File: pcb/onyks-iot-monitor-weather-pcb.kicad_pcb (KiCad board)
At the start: 2 copper layers, 100 x 82 mm, 45 parts, among them J1 53398-0371, J10 Conn_01x02_Pin, J11 Conn_01x06_Pin, J12 Conn_02x05_Odd_Even, J13 Conn_01x02_Pin, J2 53398-0371, J3 53048-0810, J3 Conn_01x04_Pin, J4 53398-0371, J5 53398-0371, J6 53398-0371, J7 53398-0371, J8 53398-0371, J9 53398-0371, Q1 SS8050, Q2 SS8050, U1 ESP32-WROOM-32D, U3 TLV75733PDBV, U6 BMP280

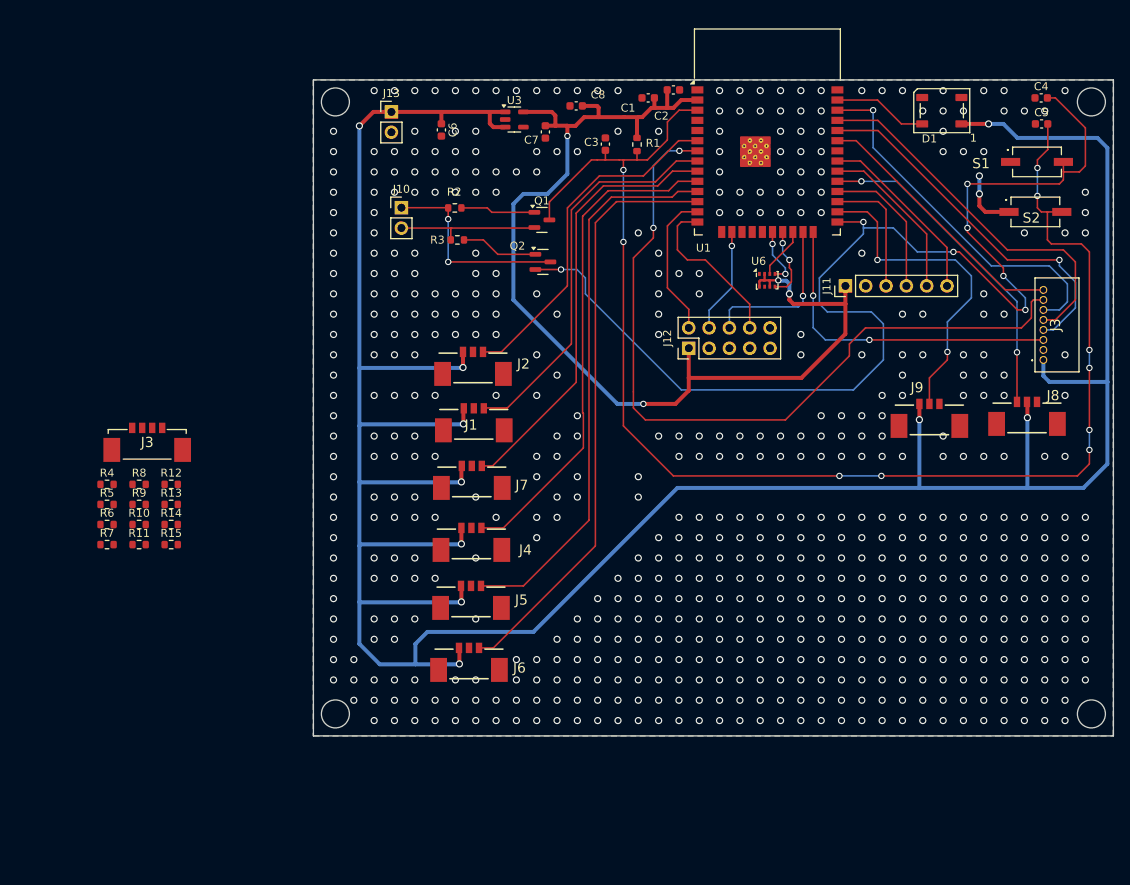
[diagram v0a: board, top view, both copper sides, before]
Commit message: zrobiony PCB
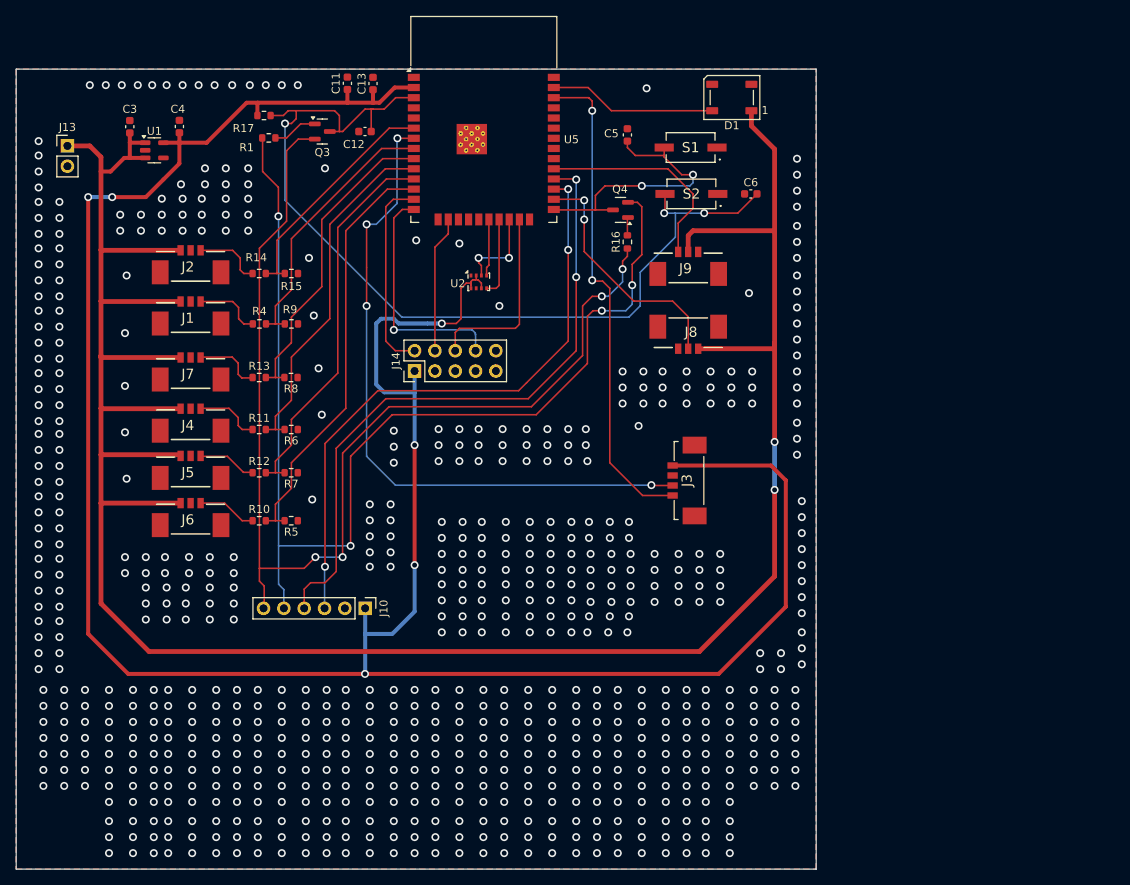
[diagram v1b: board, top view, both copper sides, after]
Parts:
- removed C1, C7, C8: 22uF/4VDC, Capacitor_SMD:C_0603_1608Metric
- removed C2: 0.1uF/4VDC, Capacitor_SMD:C_0603_1608Metric
- removed J11: Conn_01x06_Pin, Connector_PinHeader_2.54mm:PinHeader_1x06_P2.54mm_Vertical
- removed J12: Conn_02x05_Odd_Even, Connector_PinHeader_2.54mm:PinHeader_2x05_P2.54mm_Vertical
- removed the J3 at (184.0, 74.8)
- removed the J3 at (72.0, 83.5)
- removed Q1, Q2: SS8050, Package_TO_SOT_SMD:SOT-23
- removed R2, R3: 10K, Resistor_SMD:R_0603_1608Metric
- removed U3: TLV75733PDBV, Package_TO_SOT_SMD:SOT-23-5
- removed U6: BMP280, Package_LGA:Bosch_LGA-8_2x2.5mm_P0.65mm_ClockwisePinNumbering
- added C11: 22uF/10VDC, Capacitor_SMD:C_0603_1608Metric, F.Cu at (97.0, 40.2)
- added C12: 0.1uF/10VDC, Capacitor_SMD:C_0603_1608Metric, F.Cu at (99.2, 46.2)
- added C13: 0.1uF/10VDC, Capacitor_SMD:C_0603_1608Metric, F.Cu at (100.2, 40.2)
- added J14: Conn_02x05_Odd_Even, Connector_PinHeader_2.54mm:PinHeader_2x05_P2.54mm_Vertical, F.Cu at (105.4, 76.1)
- added J3: Conn_01x04_Pin, 1bmoje:533980471- MOLEXx4, F.Cu at (137.8, 89.8)
- added Q3: SS8050, Package_TO_SOT_SMD:SOT-23, F.Cu at (93.9, 46.2)
- added Q4: SS8050, Package_TO_SOT_SMD:SOT-23, F.Cu at (131.1, 56.0)
- added R16: 10K, Resistor_SMD:R_0603_1608Metric, F.Cu at (132.0, 60.0)
- added R17: 10K, Resistor_SMD:R_0603_1608Metric, F.Cu at (86.6, 44.2)
- added U2: BMP280, Package_LGA:Bosch_LGA-8_2x2.5mm_P0.65mm_ClockwisePinNumbering, F.Cu at (113.4, 65.0)
- added U5: ESP32-WROOM-32D, RF_Module:ESP32-WROOM-32D, F.Cu at (114.0, 47.7)
- C3, C4: value 0.1uF/4VDC -> 22uF/10VDC
- C6: value 22uF/4VDC -> 0.1uF/4VDC
- J10: value Conn_01x02_Pin -> Conn_01x06_Pin; footprint Connector_PinHeader_2.54mm:PinHeader_1x02_P2.54mm_Vertical -> Connector_PinHeader_2.54mm:PinHeader_1x06_P2.54mm_Vertical
- R11, R13: value 910 -> 470
- R6, R8: value 470 -> 910
- U1: value ESP32-WROOM-32D -> TLV75733PDBV; footprint RF_Module:ESP32-WROOM-32D -> Package_TO_SOT_SMD:SOT-23-5
- moved C4 107.8 mm to (76.0, 45.6), turned to 90 degrees
- moved U1 76.6 mm to (72.9, 48.5)
- moved C3 59.5 mm to (69.8, 45.6)
- moved C5 51.8 mm to (132.0, 46.6), turned to -90 degrees
- moved J10 50.3 mm to (99.2, 105.8), turned to -90 degrees
- moved R1 46.0 mm to (87.2, 47.0), turned to 0 degrees
- moved S1 43.3 mm to (139.9, 48.2), turned to 180 degrees
- moved S2 43.1 mm to (140.0, 54.0), turned to 180 degrees
- moved J8 42.9 mm to (139.6, 73.2), turned to 180 degrees
- moved J13 40.7 mm to (62.0, 48.0)
- moved C6 39.5 mm to (147.4, 54.0), turned to 0 degrees
- moved J6 39.2 mm to (77.4, 92.8)
- moved J5 38.6 mm to (77.4, 86.9)
- moved J4 38.1 mm to (77.4, 81.0)
- moved J1 37.8 mm to (77.4, 67.6)
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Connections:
- C3 pad 1: /EN -> VCC
- C4 pad 1: GND -> +3.3V
- C4 pad 2: /IO0 -> GND
- C5 pad 2: /EN -> /ESP32/IO0
- C6 pad 1: VCC -> GND
- C6 pad 2: GND -> /ESP32/EN
- D1 pad 4: /LED -> /ESP32/LED
- J10 pad 1: Net-(J10-Pin_1) -> +3.3V
- J10 pad 2: Net-(J10-Pin_2) -> GND
- J8 pad 1: /SEN0219 -> VCC
- J8 pad 2: VCC -> /ESP32/IO4
- J9 pad 1: VCC -> /ESP32/IO5
- J9 pad 2: /DHT22 -> VCC
- R1 pad 1: +3.3V -> /ESP32/UART_PROGRAM_DTR
- R1 pad 2: /EN -> Net-(Q3-B)
- R10 pad 1: Net-(J5-Pin_3) -> Net-(J6-Pin_3)
- R10 pad 2: /Hall 2 -> /ESP32/IO27
- R11 pad 1: /Hall 2 -> Net-(J4-Pin_3)
- R11 pad 2: GND -> /ESP32/IO25
- R12 pad 1: Net-(J6-Pin_3) -> Net-(J5-Pin_3)
- R12 pad 2: /Hall 3 -> /ESP32/IO26
- R13 pad 1: /Hall 3 -> Net-(J7-Pin_3)
- R13 pad 2: GND -> /ESP32/IO33
- R14 pad 1: Net-(J7-Pin_3) -> Net-(J2-Pin_3)
- R14 pad 2: /Hall 6 -> /ESP32/IO34
- R15 pad 1: /Hall 6 -> /ESP32/IO34
- R4 pad 2: /Hall 4 -> /ESP32/IO32
- R5 pad 1: /Hall 4 -> /ESP32/IO27
- R6 pad 1: Net-(J2-Pin_3) -> /ESP32/IO25
- R6 pad 2: /Hall 5 -> GND
- R7 pad 1: /Hall 5 -> /ESP32/IO26
- R8 pad 1: Net-(J4-Pin_3) -> /ESP32/IO33
- R8 pad 2: /Hall 1 -> GND
- R9 pad 1: /Hall 1 -> /ESP32/IO32
- S1 pad 2: /IO0 -> /ESP32/IO0
- S2 pad 2: /EN -> /ESP32/EN
- U1 pad 1: GND -> VCC
- U1 pad 2: +3.3V -> GND
- U1 pad 3: /EN -> VCC
- U1 pad 5: unconnected-(U1-SENSOR_VN-Pad5) -> +3.3V
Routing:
- net +3.3V: track 138.0 -> 312.7 mm, vias 4 -> 6
- net /EN: track 174.0 -> 0.00 mm, vias 10 -> 0
- net /IO0: track 153.6 -> 0.00 mm, vias 7 -> 0
- net /ESP32/UART_PROGRAM_DTR: track 0.00 -> 140.7 mm, vias 0 -> 4
- net /ESP32/UART_PROGRAM_RTS: track 0.00 -> 138.5 mm, vias 0 -> 4
- net /ESP32/EN: track 0.00 -> 118.4 mm, vias 0 -> 3
- net /PMS_PWM: track 97.7 -> 0.00 mm, vias 2 -> 0
- net /ESP32/IO35: track 0.00 -> 83.1 mm, vias 0 -> 4
- net /ESP32/UART_PROGRAM_TXD: track 0.00 -> 82.0 mm, vias 0 -> 2
- net /ESP32/UART_PROGRAM_RXD: track 0.00 -> 77.0 mm, vias 0 -> 3
- net /Hall 3: track 74.1 -> 0.00 mm
- net /Hall 2: track 69.5 -> 0.00 mm
- net /Hall 1: track 62.0 -> 0.00 mm
- net /ESP32/IO22: track 0.00 -> 61.1 mm, vias 0 -> 2
- net VCC: track 366.5 -> 305.4 mm, vias 10 -> 2
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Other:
- board size 100 x 82 mm -> 100 x 100 mm
